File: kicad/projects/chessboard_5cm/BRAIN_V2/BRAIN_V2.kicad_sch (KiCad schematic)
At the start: 64 parts, among them J1 Conn_ARM_JTAG_SWD_10, J10 Conn_01x08, J11 Conn_01x08, J2 UART, J3 USB_C_Receptacle_USB2.0_16P, J4 Conn_02x06_Odd_Even, J5 I2C, J6 Conn_01x08, J7 Conn_02x04_Odd_Even, J8 Conn_01x08, J9 USB_C_Receptacle_USB2.0_16P, Q1 BC847, SW1 TL3342F450QG, U1 24LC512, U3 AP2112K-3.3, U4 AP2112K-3.3, U73 STM32L433CCTx

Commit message: brain completed
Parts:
- removed J10, J11, J6, J8: Conn_01x08, Connector_PinSocket_2.54mm:PinSocket_1x08_P2.54mm_Horizontal, symbol Connector_Generic:Conn_01x08
- added C2, C3: 100nF, Capacitor_SMD:C_0805_2012Metric_Pad1.18x1.45mm_HandSolder, symbol Device:C
- added J6: HCTL PM254-1-13-W-8.5, Connector_PinSocket_2.54mm:PinSocket_1x13_P2.54mm_Horizontal, symbol Connector_Generic:Conn_01x13
- added J8: Conn_01x02, Connector_PinHeader_2.54mm:PinHeader_1x02_P2.54mm_Vertical, symbol Connector_Generic:Conn_01x02
- added R18, R19, R24: 10k, Resistor_SMD:R_0805_2012Metric_Pad1.20x1.40mm_HandSolder, symbol Device:R
- added SW2, SW3: TS-1187A-B-A-B, Button_Switch_SMD:SW_SPST_TL3342, symbol Switch:SW_Push
- C1, C16, C6: MANUFACTURER (none) -> CL21B104KBCNNNC
- C10, C11, C8, C9: LCSC p/n C28323 -> C24123; MANUFACTURER (none) -> CL21B105KOFNNNE; shop https://www.lcsc.com/product-detail/Multilayer-Ceramic-Capacitors-MLCC-SMD-SMT_Samsung-Electro-Mechanics-CL21B105KBFNNNE_C28323.html?s_z=n_1uF -> https://www.lcsc.com/product-detail/Multilayer-Ceramic-Capacitors-MLCC-SMD-SMT_Samsung-Electro-Mechanics-CL21B105KOFNNNE_C24123.html?s_z=n_CL21A105KOFNNNE
- C12, C13, C14, C15, C5: MANUFACTURER (none) -> CL21B105KOFNNNE
- C4, C7: MANUFACTURER (none) -> 0805CG4R7C500NT
- D1, D3, D9: MANUFACTURER (none) -> NCD0805G1
- D10: MANUFACTURER (none) -> PESD5V0L2BT,215
- D2: MANUFACTURER (none) -> TVS3V3L4U
- D4, D5: MANUFACTURER (none) -> SS14-E3/61T
- D6: MANUFACTURER (none) -> NCD0805R1
- D8: MANUFACTURER (none) -> XL-2012UBC
- J1: MANUFACTURER (none) -> BD125-16-A-0305-0580-L-B
- J2: value UART -> C2691448; MANUFACTURER (none) -> PZ254V-11-04P
- J3, J9: MANUFACTURER (none) -> U262-161N-4BS165
- J4: value Conn_02x06_Odd_Even -> HCTL PM254-2-06-S-8.5; LCSC p/n (none) -> C3975151; MANUFACTURER (none) -> PM254-2-06-S-8.5; shop (none) -> https://www.lcsc.com/product-detail/C3975151.html?s_z=n_q_P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
- J5: value I2C -> C2691448; MANUFACTURER (none) -> PZ254V-11-04P
- J7: value Conn_02x04_Odd_Even -> HCTL PM254-2-04-S-8.5; LCSC p/n (none) -> C3975149; MANUFACTURER (none) -> PM254-2-04-S-8.5; shop (none) -> https://www.lcsc.com/product-detail/C3975149.html?s_z=n_q_H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
- LS1: LCSC p/n (none) -> C3811958; MANUFACTURER CUI INC -> CMT-1203-SMT-TR
- Q1: MANUFACTURER (none) -> MMBT4401LT1G
- R1: MANUFACTURER (none) -> RC0805FR-071KL
- R10, R11, R12, R15, R16, R17, R7, R8, R9: MANUFACTURER (none) -> RC0805FR-075K1L
- R13: LCSC p/n (none) -> C100045; MANUFACTURER (none) -> RC0805FR-070RL; shop (none) -> https://www.lcsc.com/product-detail/C100045.html?s_z=n_q_RC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
- R14, R20, R21, R22, R23, R26: MANUFACTURER (none) -> RC0805FR-0710KL
- R27: LCSC p/n (none) -> C96346; MANUFACTURER (none) -> RC0805FR-07100KL; shop (none) -> https://www.lcsc.com/product-detail/C96346.html?s_z=n_q_RC0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
- R3, R4, R5, R6: MANUFACTURER (none) -> 0805W8F1000T5E
- SW1: value TL3342F450QG -> TS-1187A-B-A-B; MANUFACTURER (none) -> TS-1187A-B-A-B
- U1: MANUFACTURER (none) -> 24LC512T-I/SN
- U3, U4: MANUFACTURER (none) -> AP2112K-3.3TRG1
- U73: LCSC p/n (none) -> C110061; MANUFACTURER (none) -> STM32L433CCT6; shop (none) -> https://www.lcsc.com/product-detail/C110061.html?s_z=n_q_p_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
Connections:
- net +3V3: now also R18.1, R19.1, R24.1
- net 3V3_OUT: now also J6.13 (Pin_13), J6.2 (Pin_2)
- net GND: now also C2.1, C3.1, J6.1 (Pin_1), J6.3 (Pin_3), J6.8 (Pin_8), J8.2 (Pin_2), SW2.1, SW3.1
- net MUX1: now also J6.9 (Pin_9)
- net MUX2: now also J6.10 (Pin_10)
- net MUX3: now also J6.11 (Pin_11)
- net MUX4: now also J6.12 (Pin_12)
- net SIG1: now also R3.1, J6.4 (Pin_4); no longer R6.1
- net SIG2: now also R4.1, J6.5 (Pin_5); no longer R5.1
- net SIG3: now also R5.1, J6.6 (Pin_6); no longer R4.1
- net SIG4: now also R6.1, J6.7 (Pin_7); no longer R3.1
- net SW_USER1: now reaches U73.10 (PA0)
- net SW_USER1: now also C2.2, R18.2, SW2.2
- net JUMPER: now reaches U73.44 (PH3)
- net JUMPER: now also J8.1 (Pin_1), R24.2
- net SW_USER2: now reaches U73.6 (PH1)
- net SW_USER2: now also C3.2, R19.2, SW3.2
- no-connect marks 14 -> 11

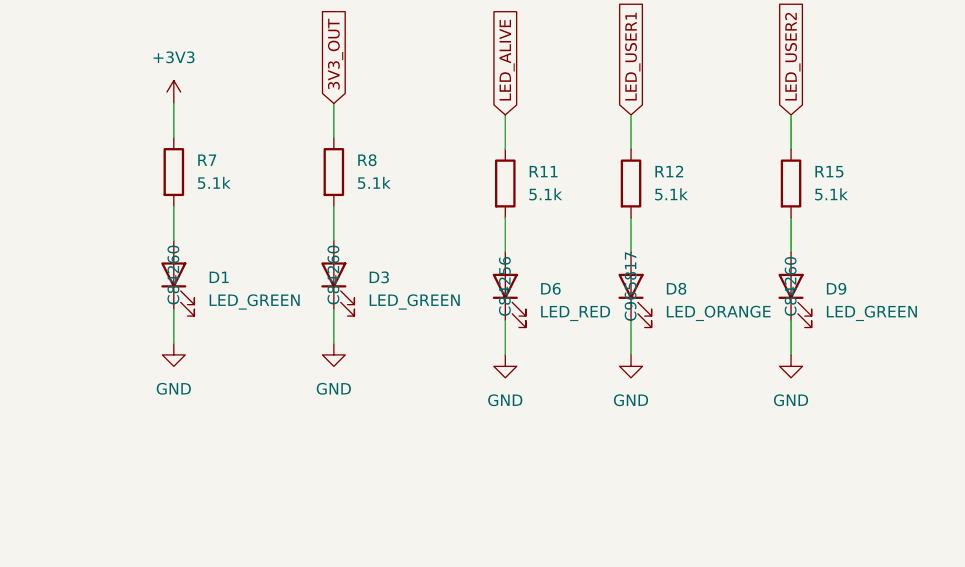
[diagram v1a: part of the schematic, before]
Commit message: brain changes. all components at top and started to change into basic comps
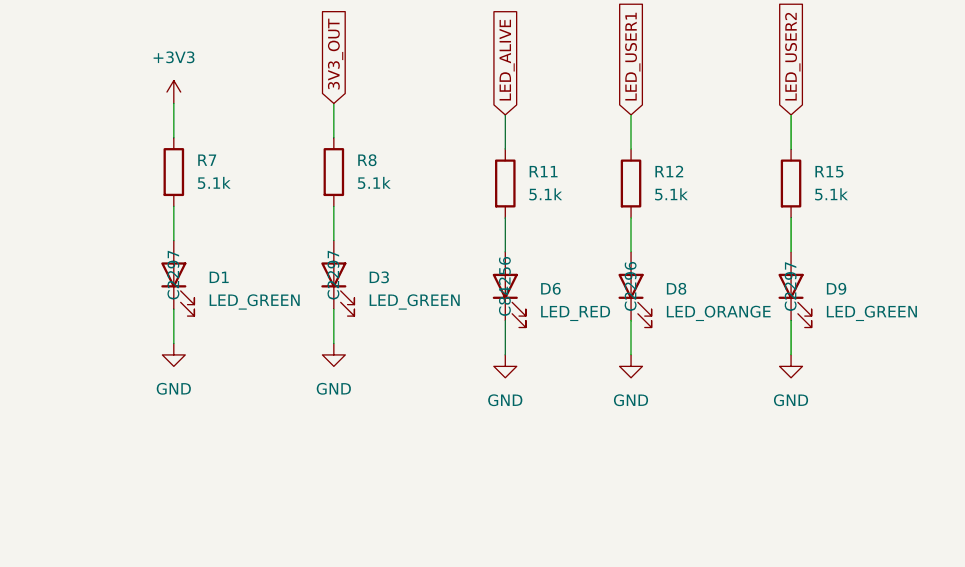
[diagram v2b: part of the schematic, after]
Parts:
- D1, D3, D9: LCSC p/n C84260 -> C2297; MANUFACTURER NCD0805G1 -> KT-0805G; shop https://www.lcsc.com/product-detail/LED-Indication-Discrete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 -> https://www.lcsc.com/product-detail/C2296.html?s_z=n_q_C229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
- D8: LCSC p/n C965817 -> C2296; MANUFACTURER XL-2012UBC -> KT-0805Y
- Q1: shop https://www.lcsc.com/product-detail/Bipolar-BJT_onsemi-MMBT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 -> (none)
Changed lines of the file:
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@@
 			)
 		)
-		(property "shop" "https://www.lcsc.com/product-detail/LED-Indication-Discrete_Foshan-NationStar-Optoelectronics-NCD0805G1_C84260.html"
+		(property "shop" "https://www.lcsc.com/product-detail/C2296.html?s_z=n_q_C2296&globalKeyword=C2296"
 			(at 201.93 67.31 0)
 			(effects
@@
 			)
 		)
-		(property "LCSC p/n" "C84260"
+		(property "LCSC p/n" "C2297"
 			(at 201.93 67.31 0)
 			(effects
@@
 			)
 		)
-		(property "MANUFACTURER" "NCD0805G1"
+		(property "MANUFACTURER" "KT-0805G"
 			(at 201.93 67.31 90)
 			(effects
@@
 			)
 		)
-		(property "shop" "https://www.lcsc.com/product-detail/LED-Indication-Discrete_Foshan-NationStar-Optoelectronics-NCD0805G1_C84260.html"
+		(property "shop" "https://www.lcsc.com/product-detail/C2296.html?s_z=n_q_C2296&globalKeyword=C2296"
 			(at 270.51 68.58 0)
 			(effects
@@
 			)
 		)
-		(property "LCSC p/n" "C84260"
+		(property "LCSC p/n" "C2297"
 			(at 270.51 68.58 0)
 			(effects
@@
 			)
 		)
-		(property "MANUFACTURER" "NCD0805G1"
+		(property "MANUFACTURER" "KT-0805G"
 			(at 270.51 68.58 90)
 			(effects
@@
 			)
 		)
-		(property "shop" "https://www.lcsc.com/product-detail/LED-Indication-Discrete_Foshan-NationStar-Optoelectronics-NCD0805G1_C84260.html"
+		(property "shop" "https://www.lcsc.com/product-detail/C2296.html?s_z=n_q_C2296&globalKeyword=C2296"
 			(at 219.71 67.31 0)
 			(effects
@@
 			)
 		)
-		(property "LCSC p/n" "C84260"
+		(property "LCSC p/n" "C2297"
 			(at 219.71 67.31 0)
 			(effects
@@
 			)
 		)
-		(property "MANUFACTURER" "NCD0805G1"
+		(property "MANUFACTURER" "KT-0805G"
 			(at 219.71 67.31 90)
 			(effects
@@
 			)
 		)
-		(property "Datasheet" "http://www.infineon.com/dgdl/Infineon-BC847SERIES_BC848SERIES_BC849SERIES_BC850SERIES-DS-v01_01-en.pdf?fileId=db3a304314dca389011541d4630a1657"
+		(property "Datasheet" "https://jlc-prod-smt.oss-eu-central-1.aliyuncs.com/smtDataManualFile/8639582106218377216-C2297.pdf?response-content-disposition=attachment%3B%20filename%3DC2297.pdf%3B%20filename%2A%3DUTF-8%27%27C2297.pdf&x-oss-date=20261028T225704Z&x-oss-expires=1800&x-oss-security-token=CAISgAN1q6Ft5B2yfSjIr5nCGd7Ah4dk1beDW1z2gGohddhpgKrIkjz2IHhMdHJsAOodtv0%2FmmhT6PkclqRLcbhpcmfjV%2BZHzLB8qdl76kox557b16cNrbH4M4H6aXeirtuwDsz9SNTCALjPD3nPii50x5bjaDymRCbLGJaViJlhHLN1Ow6jdmhpCctxLAlvo9NgFxm3D%2Fu2NQPwiWf9FVdhvhEG6Vly8qOi2MaRmFy8yFTx0b0SvJ%2BjYMrmPctoN9JnSdC5mfdzau3a1TJ84gRD0a5wkaVA1zbDs5bfISEIuUzebreLqY03dV4mOvdqIcMe8qigz88fk%2FfIioH6xyxKOexoSCnFTOiiupCcQLPyao9jLu6iayqViY7QaIOTqQohZmkAMwVOasAsI3Ngh4zF97Qt0cVNkXO9gWfLI8DtuMleWirpxNhSjJSgc5lCkRRYwGs1287ugXlSQzo890KPDAEovaKCnZ2ZSfh7Y4sNknI6i%2Bfc2Se2MIkIpDrBWaKWD5sagAGiLi8TLKkbwmlm7pISy8%2FkVataWJ1%2FHw%2BjURyel9EVGwLwRjOqwBdeJnzUsvykwW%2FhmoSW91igTHMS0ZohG9gqTFQlhCqkVgrgS1JyQX2RCNwdnQZHPWIxaGE6chQei0mdbREVl7GbZv9m9NtkvRanFtZsUXmMxTSjfMpDGqzP%2FCAA&x-oss-signature-version=OSS4-HMAC-SHA256&x-oss-credential=STS.NZwRdtjXEbuhYzGdjtyWEoocp%2F20261028%2Feu-central-1%2Foss%2Faliyun_v4_request&x-oss-signature=b23b426dad90a518e6dbc62cc78fc666dfb630e1c3cb827b7a5714bf1062451c"
 			(at 114.3 139.7 0)
 			(effects
@@
 			)
 		)
-		(property "shop" "https://www.lcsc.com/product-detail/Bipolar-BJT_onsemi-MMBT4401LT1G_C31776.html"
+		(property "shop" ""
 			(at 114.3 139.7 0)
 			(effects
@@
 			)
 		)
-		(property "LCSC p/n" "C965817"
+		(property "LCSC p/n" "C2296"
 			(at 252.73 68.58 0)
 			(effects
@@
 			)
 		)
-		(property "MANUFACTURER" "XL-2012UBC"
+		(property "MANUFACTURER" "KT-0805Y"
 			(at 252.73 68.58 90)
 			(effects
